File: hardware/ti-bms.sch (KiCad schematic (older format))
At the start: 48 parts, among them J1 Conn_02x04_Odd_Even, J2 Conn_02x03_Odd_Even, J4 CAN_TERM, Q1 NCV8402xST, U1 Pico, U2 MCP2515-xST, U3 SN65HVD230, U4 TPS62160DGK, U5 MAX3485, U6 MAX3485

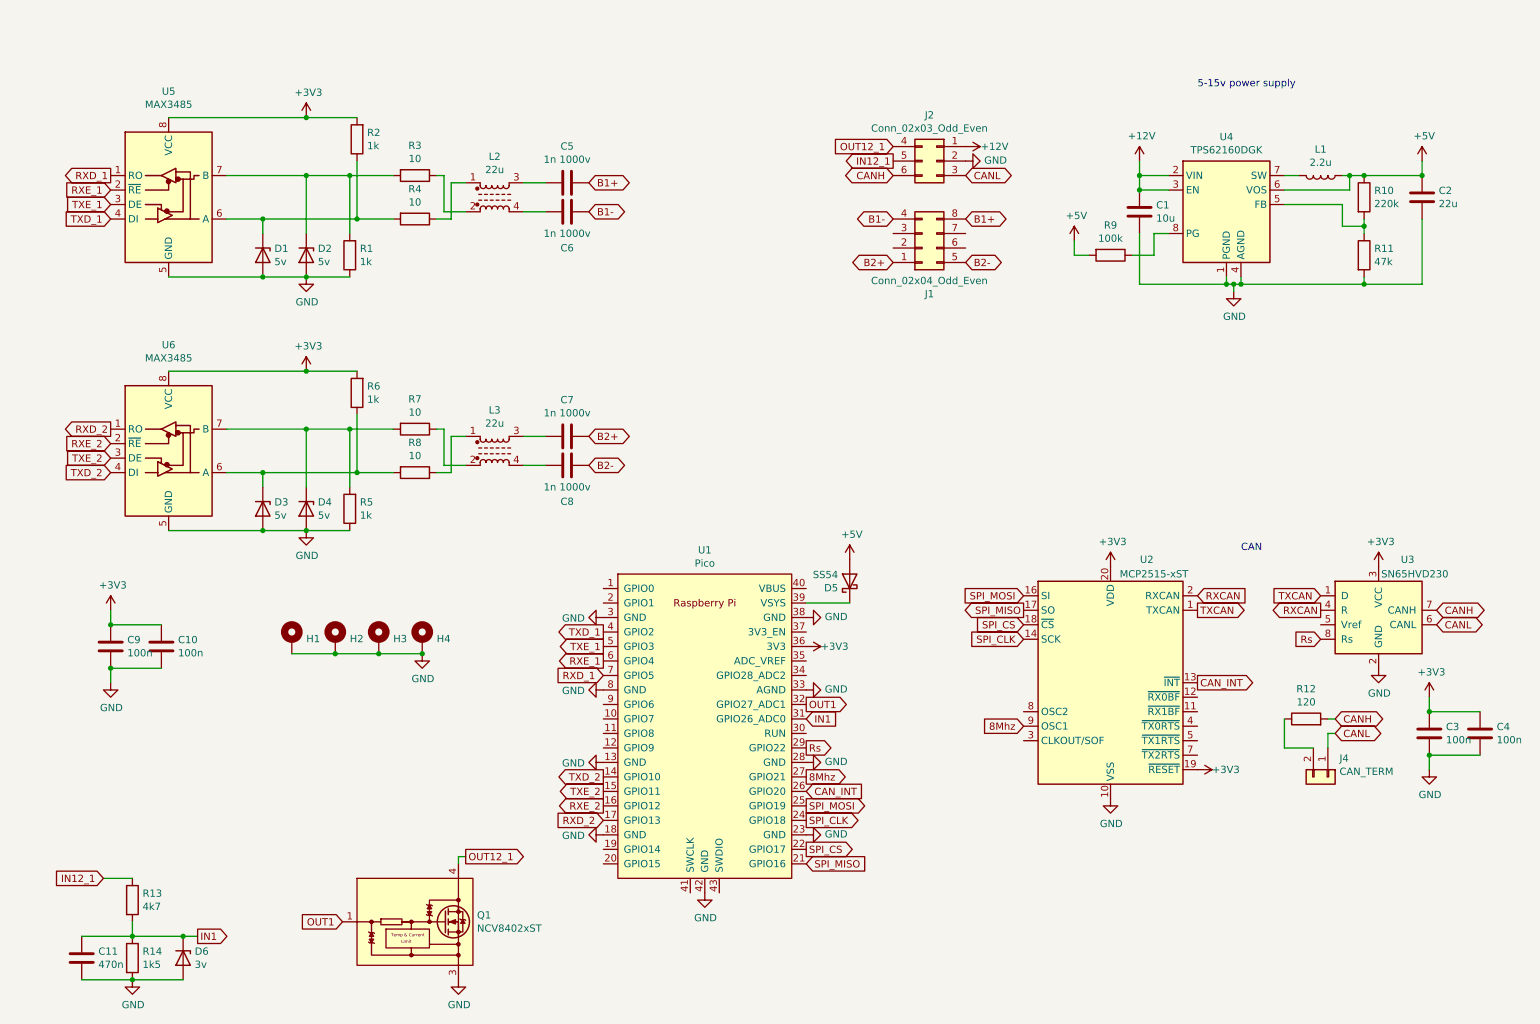
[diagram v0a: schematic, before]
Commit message: v3
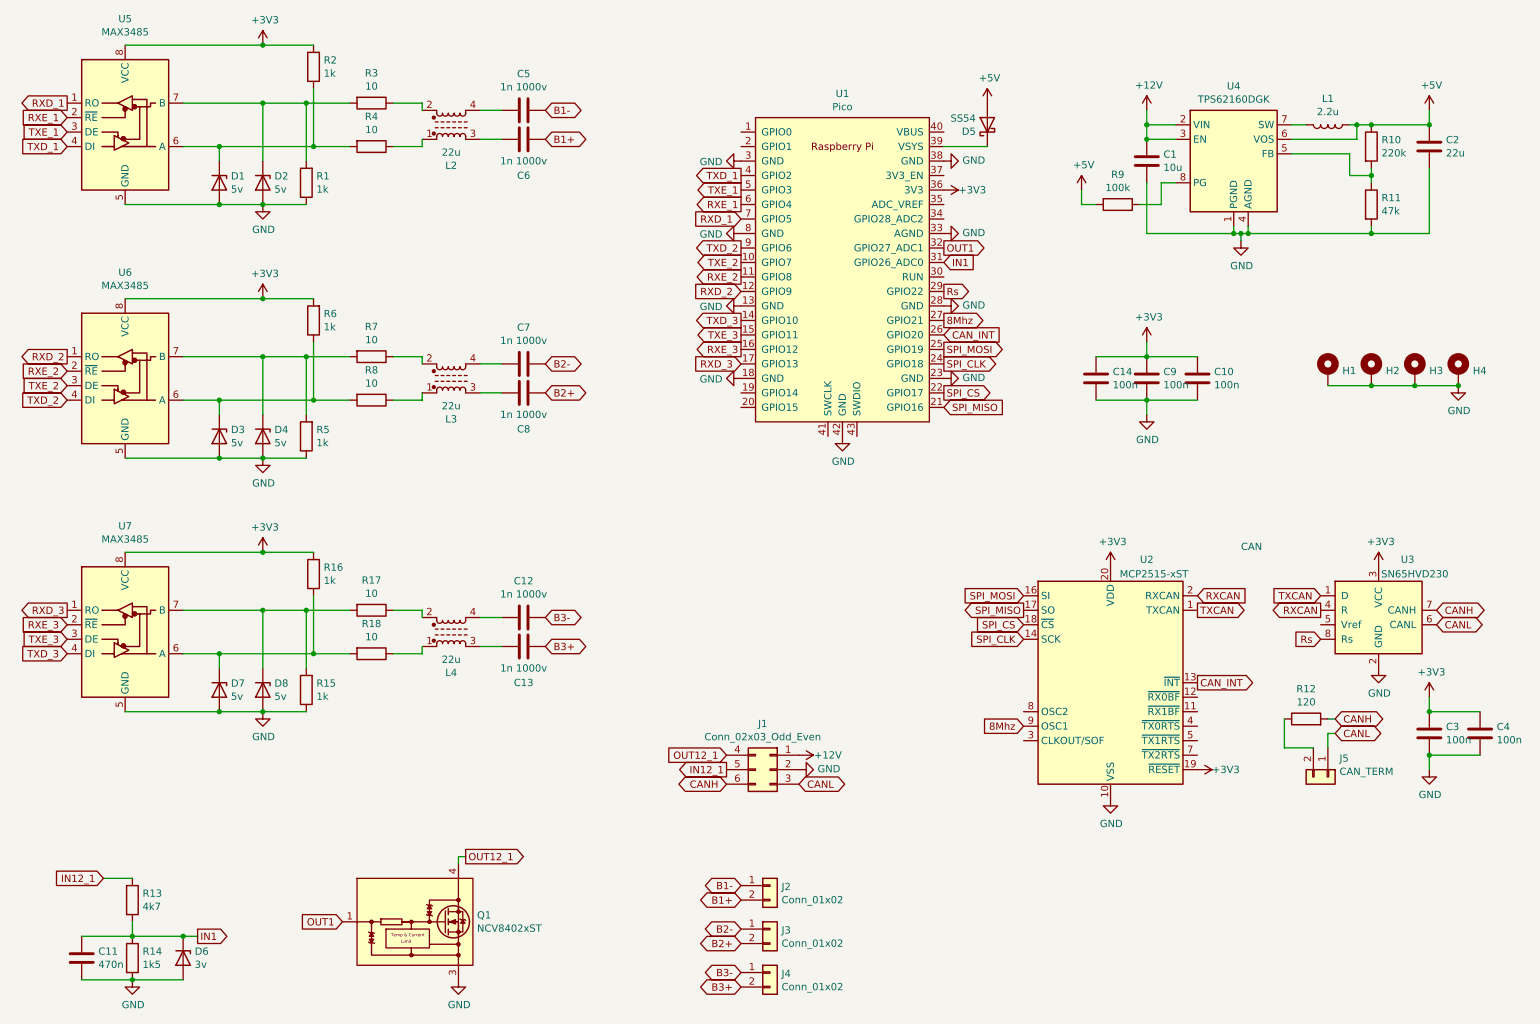
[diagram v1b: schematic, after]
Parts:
- removed J1: Conn_02x04_Odd_Even, Connector_Molex:Molex_Micro-Fit_3.0_43045-0800_2x04_P3.00mm_Horizontal, symbol Connector_Generic:Conn_02x04_Top_Bottom
- added C12, C13: 1n 1000v, Capacitor_SMD:C_1206_3216Metric, symbol Device:C
- added C14: 100n, Capacitor_SMD:C_0603_1608Metric, symbol Device:C
- added D7, D8: 5v, footprints:SOD882, symbol Device:D_Zener
- added J2, J3, J4: Conn_01x02, Connector_Molex:Molex_Micro-Fit_3.0_43650-0200_1x02_P3.00mm_Horizontal, symbol Connector_Generic:Conn_01x02
- added L4: 22u, footprints:ACT45B-101-2P-TL003, symbol Device:L_Core_Ferrite_Coupled_1324
- added R15, R16: 1k, Resistor_SMD:R_0603_1608Metric, symbol Device:R
- added R17, R18: 10, Resistor_SMD:R_0603_1608Metric, symbol Device:R
- added U7: MAX3485, Package_SO:SOP-8_3.9x4.9mm_P1.27mm, symbol Interface_UART:MAX3485
- renumbered J2 to J1, J4 to J5
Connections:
- net +3V3: now also C14.1, R16.2, U7.8 (VCC)
- net B1+: now also C6.1, J2.2 (Pin_2); no longer C5.1
- net B1-: now also C5.1, J2.1 (Pin_1); no longer C6.1
- net B2+: now also C8.1, J3.2 (Pin_2); no longer C7.1
- net B2-: now also C7.1, J3.1 (Pin_1); no longer C8.1
- net GND: now also C14.2, D7.2 (A), D8.2 (A), R15.1, U7.5 (GND)
- net RXD_2: now also U1.12 (GPIO9); no longer U1.17 (GPIO13)
- net RXE_2: now also U1.11 (GPIO8); no longer U1.16 (GPIO12)
- net TXD_2: now also U1.9 (GPIO6); no longer U1.14 (GPIO10)
- net TXE_2: now also U1.10 (GPIO7); no longer U1.15 (GPIO11)
- net at L2.3: now also C6.2; no longer C5.2
- net at L2.4: now also C5.2; no longer C6.2
- net at L3.3: now also C8.2; no longer C7.2
- net at L3.4: now also C7.2; no longer C8.2
- new net: D7.1 (K), R16.1, R18.2, U7.6 (A)
- new net: D8.1 (K), R15.2, R17.2, U7.7 (B)
- new net: L4.2, R17.1
- new net: L4.1, R18.1
- new net: C13.2, L4.3
- new net: C12.2, L4.4
- new net B3+: C13.1, J4.2 (Pin_2)
- new net B3-: C12.1, J4.1 (Pin_1)
- new net RXD_3: U1.17 (GPIO13), U7.1 (RO)
- new net RXE_3: U1.16 (GPIO12), U7.2 (~RE)
- new net TXD_3: U1.14 (GPIO10), U7.4 (DI)
- new net TXE_3: U1.15 (GPIO11), U7.3 (DE)
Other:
- note removed: "5-15v power supply"
- moved on the sheet: C1, C10, C2, C5, C6, C7, C8, C9, D1, D2, D3, D4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
